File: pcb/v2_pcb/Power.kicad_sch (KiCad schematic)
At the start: 41 parts, among them Q3 NMOS, Q4 NMOS, Q5 NMOS, U6 BQ25798RQMR, U7 MAX17320G22+

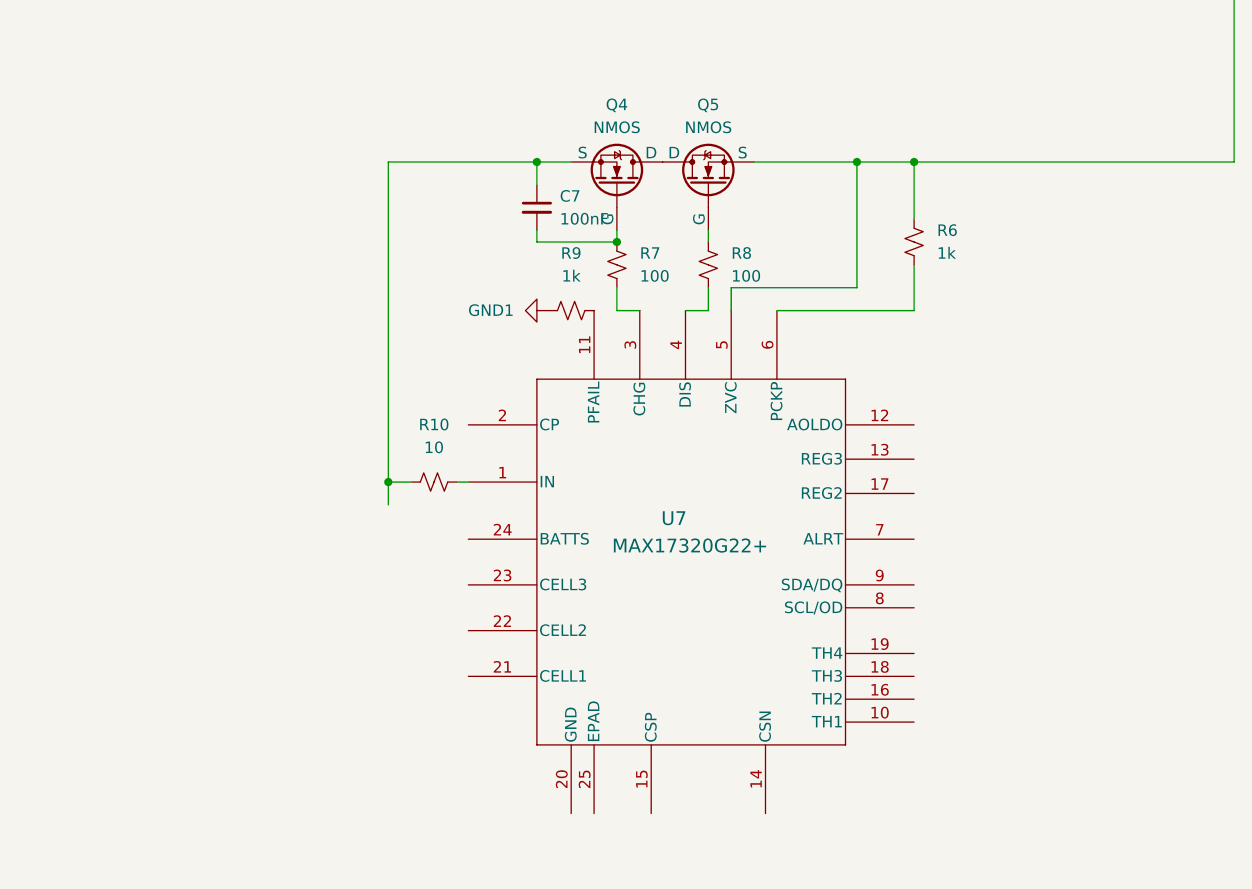
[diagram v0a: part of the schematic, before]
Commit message: fnish micro sd card
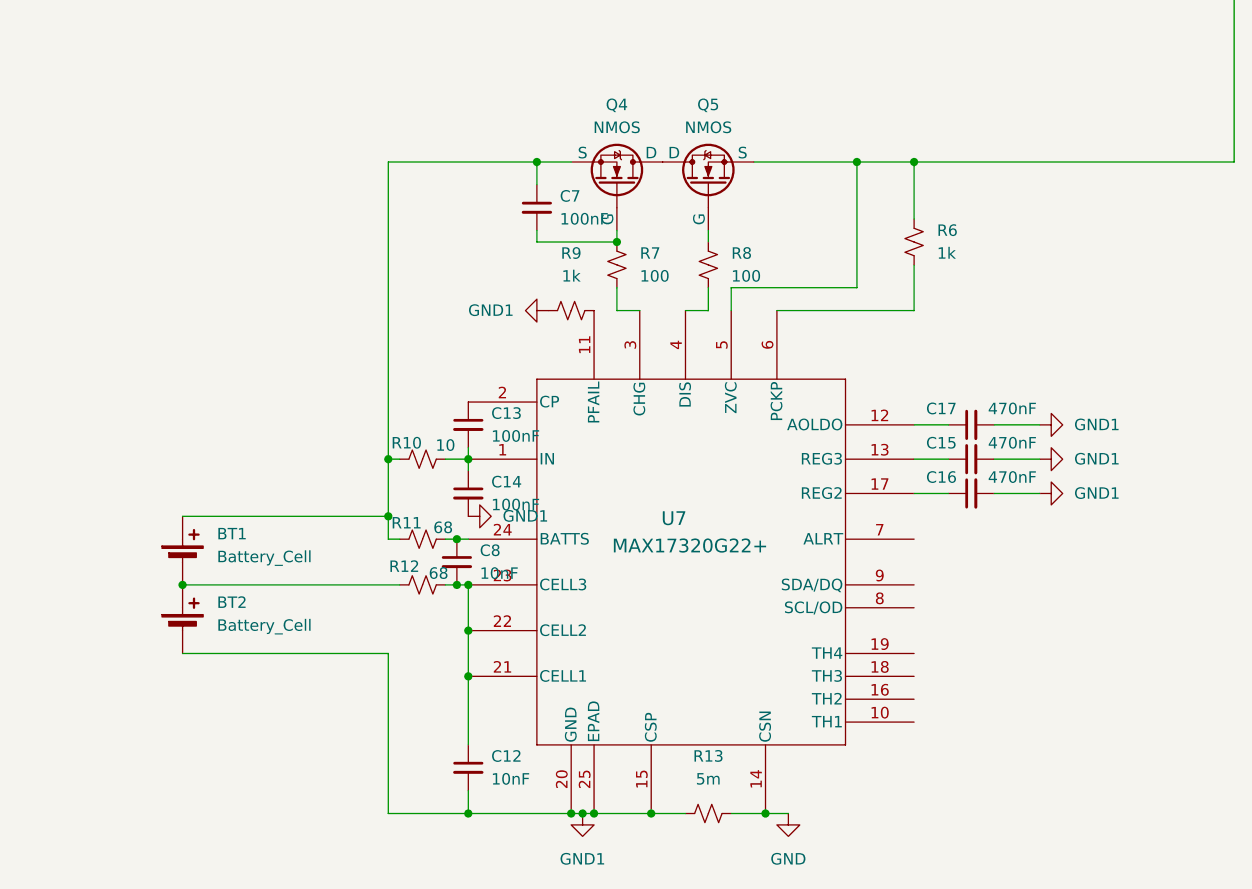
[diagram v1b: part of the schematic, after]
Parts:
- added BT1, BT2: Battery_Cell, symbol Device:Battery_Cell
- added C12, C8: 10nF, symbol Device:C_Small
- added C13, C14: 100nF, symbol Device:C_Small
- added C15, C16, C17: 470nF, symbol Device:C_Small
- added R11, R12: 68, symbol Device:R_Small_US
- added R13: 5m, symbol Device:R_Small_US
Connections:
- net GND: now also U7.14 (CSN), R13.2
- net GND1: now also U7.15 (CSP), U7.20 (GND), U7.25 (EPAD), BT2.2 (-), C12.2, C14.2, C15.2, C16.2, C17.2, R13.1
- net at R10.2, U7.1 (IN): now also C13.2, C14.1
- net at U7.12 (AOLDO): now also C17.1
- net at U7.13 (REG3): now also C15.1
- net at U7.17 (REG2): now also C16.1
- net at U7.2 (CP): now also C13.1
- net at U7.21 (CELL1): now also U7.22 (CELL2), U7.23 (CELL3), C12.1, C8.2, R12.2
- net at U7.24 (BATTS): now also C8.1, R11.2
- net at C7.1, Q4.3 (S), R10.1: now also BT1.1 (+), R11.1
- new net: BT1.2 (-), BT2.1 (+), R12.1
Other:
- moved on the sheet: R10
